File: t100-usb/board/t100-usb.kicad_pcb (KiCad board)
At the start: 2 copper layers, 34.5 x 99.5 mm, 36 parts, among them J1 Conn_01x02_Female, J2 USB_B_Micro, J3 T100-OUT, U1 FR8205, U2 FR8205, U3 ATSAMD11C14A-SS, X1 SWD

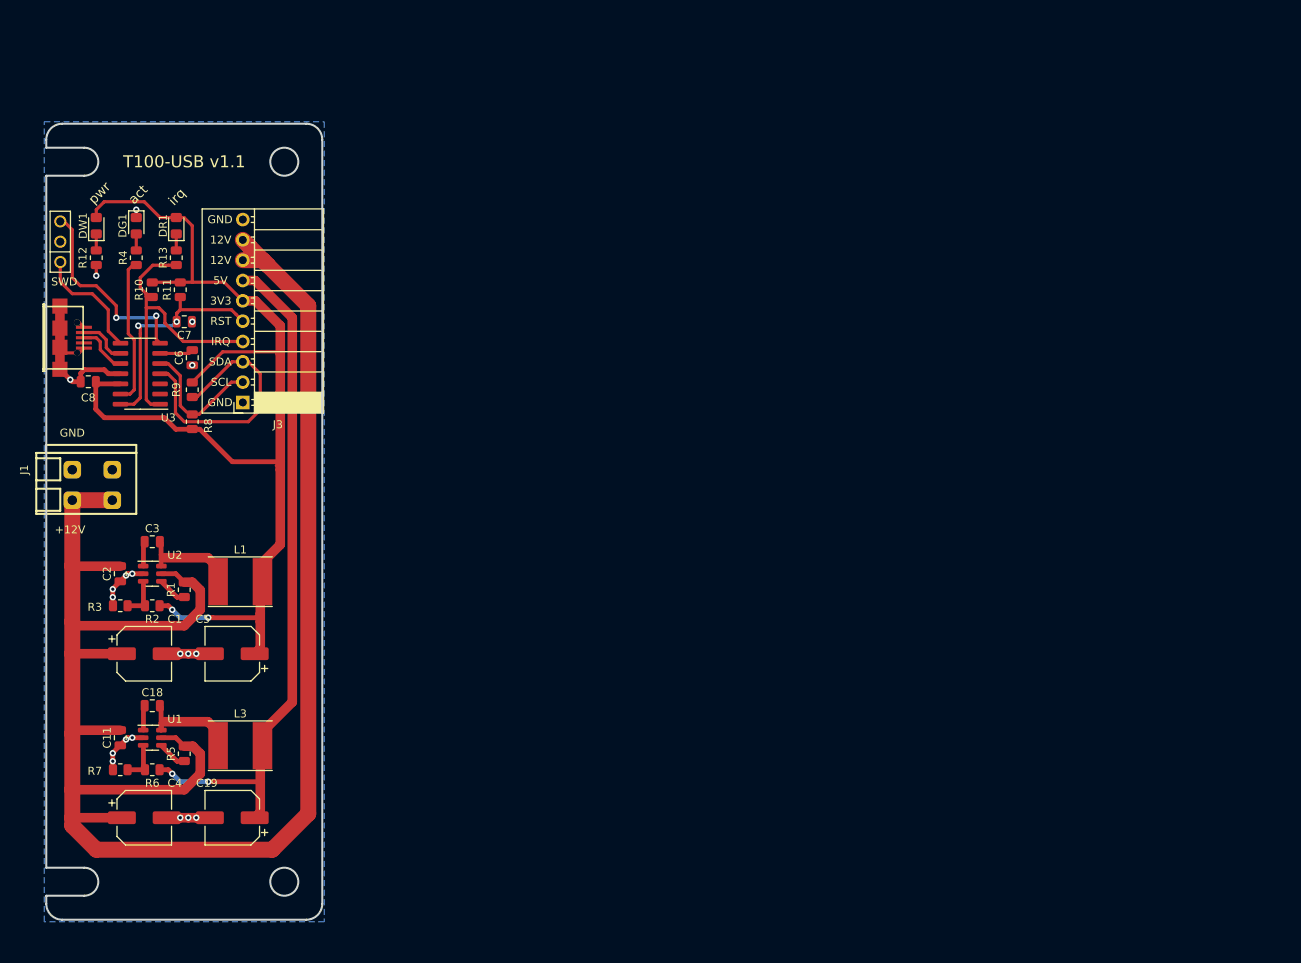
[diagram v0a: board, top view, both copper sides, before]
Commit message: WIP
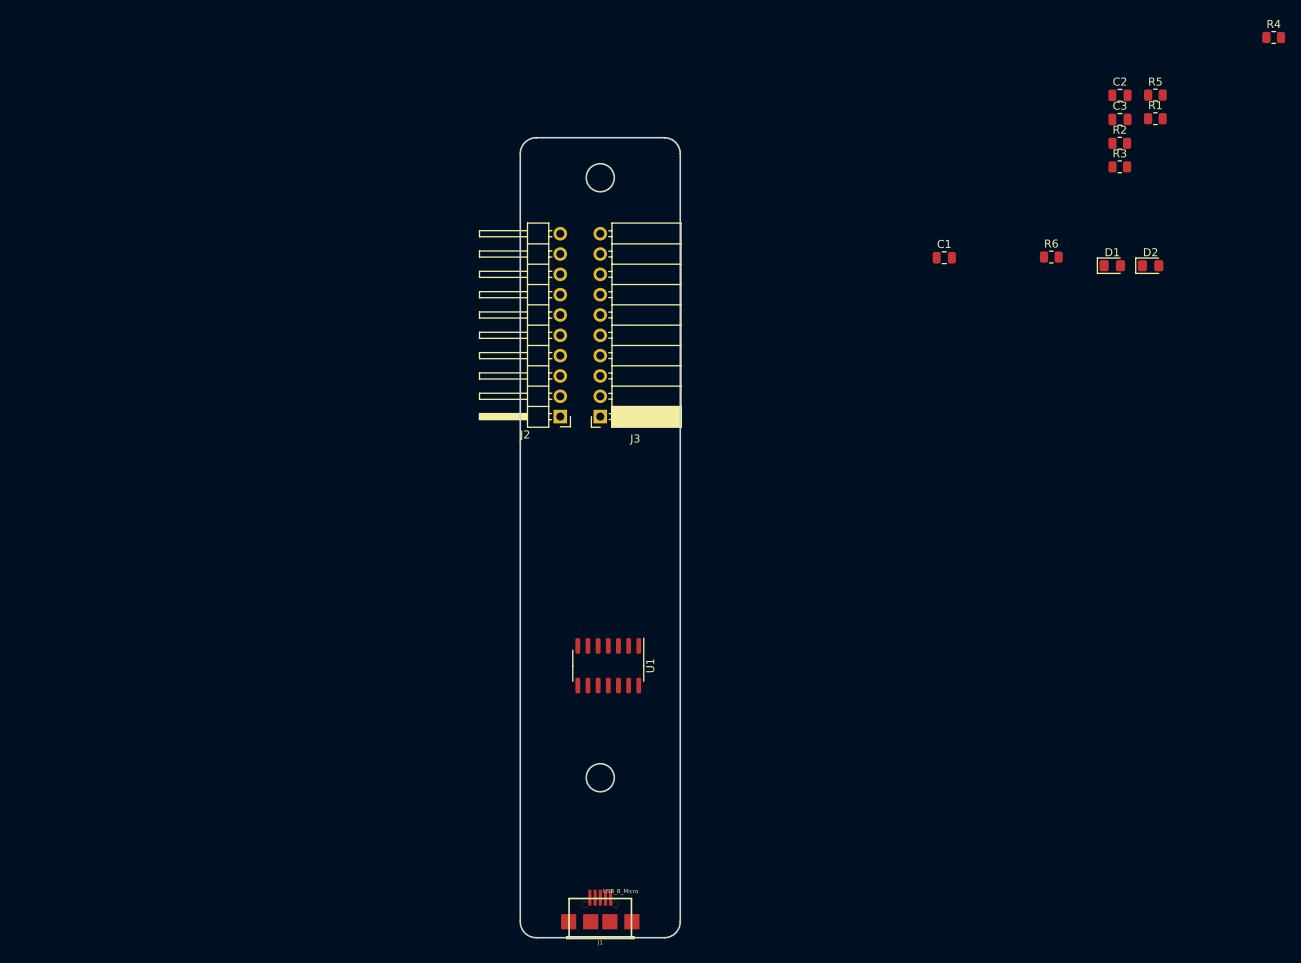
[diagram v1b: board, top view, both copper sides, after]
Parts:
- removed C11, C18, C6, C7, C8: 100n, Capacitor_SMD:C_0805_2012Metric
- removed C19, C4, C5: 100u/12V, Capacitor_SMD:CP_Elec_6.3x5.4
- removed DG1: GREEN, LED_SMD:LED_0805_2012Metric_Pad1.15x1.40mm_HandSolder
- removed DR1: RED, LED_SMD:LED_0805_2012Metric_Pad1.15x1.40mm_HandSolder
- removed DW1: WHITE, LED_SMD:LED_0805_2012Metric_Pad1.15x1.40mm_HandSolder
- removed L1, L3: 6.8uH, Drake:CKCS6028
- removed R10, R11, R8, R9: 1K5, Resistor_SMD:R_0805_2012Metric
- removed R12: 1k5, Resistor_SMD:R_0805_2012Metric
- removed R13: 270R, Resistor_SMD:R_0805_2012Metric
- removed R7: 4.22k 1%, Resistor_SMD:R_0805_2012Metric
- removed U2: FR8205, Package_TO_SOT_SMD:SOT-23-6
- removed U3: ATSAMD11C14A-SS, Package_SO:SOIC-14_3.9x8.7mm_P1.27mm
- removed X1: SWD, Drake:SWD
- added D1: GREEN, LED_SMD:LED_0805_2012Metric_Pad1.15x1.40mm_HandSolder, F.Cu at (216.0, 68.0)
- added D2: RED, LED_SMD:LED_0805_2012Metric_Pad1.15x1.40mm_HandSolder, F.Cu at (220.8, 68.0)
- C1: value 100u/12V -> 100n; footprint Capacitor_SMD:CP_Elec_6.3x5.4 -> Capacitor_SMD:C_0805_2012Metric
- J1: value Conn_01x02_Female -> USB_B_Micro; footprint Drake:DG235-3.81-02P -> Drake:conn_usb_B_micro_smd-2
- J2: value USB_B_Micro -> T100-IN; footprint Drake:conn_usb_B_micro_smd-2 -> Connector_PinHeader_2.54mm:PinHeader_1x10_P2.54mm_Horizontal
- R1: value 100k -> 1K5
- R2: value 30k 1% -> 1K5
- R3: value 6.65k 1% -> 1K5
- R4: value 270R -> 1K5
- R5: value 100k -> 270R
- R6: value 30.9k 1% -> 270R
- U1: value FR8205 -> ATSAMD11C14A-SS; footprint Package_TO_SOT_SMD:SOT-23-6 -> Package_SO:SOIC-14_3.9x8.7mm_P1.27mm
- moved R5 146.7 mm to (221.4, 46.7), turned to 0 degrees
- moved R4 144.8 mm to (236.2, 39.5), turned to 0 degrees
- moved C2 138.5 mm to (217.0, 46.7), turned to 0 degrees
- moved R3 136.5 mm to (216.9, 55.6)
- moved R1 134.9 mm to (221.4, 49.6), turned to 0 degrees
- moved R2 134.0 mm to (216.9, 52.7)
- moved C3 132.0 mm to (217.0, 49.7)
- moved R6 129.4 mm to (208.4, 66.9)
- moved C1 111.6 mm to (195.0, 67.0)
- moved J1 83.1 mm to (152.0, 150.0), turned to 0 degrees
- moved J2 63.3 mm to (147.0, 86.9), turned to 180 degrees
- moved U1 57.7 mm to (153.0, 118.0), turned to -90 degrees
- moved J3 44.7 mm to (152.0, 86.9)
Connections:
- C1 pad 1: +12V -> GND
- C1 pad 2: GND -> +3V3
- C2 pad 2: +12V -> Net-(C2-Pad2)
- C3 pad 1: Net-(C3-Pad1) -> GND
- C3 pad 2: Net-(C3-Pad2) -> /RST
- J1 pad 1: GND -> unconnected-(J1-Pad1)
- J1 pad 2: +12V -> /USB_DM
- J2 pad 1: unconnected-(J2-Pad1) -> GND
- J2 pad 2: /USB_DM -> /SCL
- J2 pad 3: /USB_DP -> /SDA
- J2 pad 4: unconnected-(J2-Pad4) -> /IRQ
- J2 pad 5: GND -> /RST
- J2 pad 6: GND -> +3V3
- R1 pad 1: Net-(R1-Pad1) -> /SCL
- R1 pad 2: +12V -> +3V3
- R2 pad 1: Net-(R2-Pad1) -> /SDA
- R3 pad 1: GND -> /IRQ
- R3 pad 2: Net-(R2-Pad1) -> +3V3
- R4 pad 1: /I2C_ACT -> /RST
- R4 pad 2: Net-(DG1-Pad2) -> +3V3
- R5 pad 1: Net-(R5-Pad1) -> /I2C_ACT
- R5 pad 2: +12V -> Net-(D1-Pad2)
- R6 pad 1: Net-(R6-Pad1) -> /IRQ
- R6 pad 2: +5V -> Net-(D2-Pad1)
- U1 pad 1: Net-(C18-Pad1) -> /IRQ
- U1 pad 2: GND -> unconnected-(U1-Pad2)
- U1 pad 3: Net-(R6-Pad1) -> unconnected-(U1-Pad3)
- U1 pad 4: Net-(R5-Pad1) -> /SDA
- U1 pad 5: +12V -> /SCL
- U1 pad 6: Net-(C18-Pad2) -> Net-(C2-Pad2)
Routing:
- net +12V: track 231.8 -> 0.00 mm
- net +3V3: track 141.5 -> 0.00 mm, vias 2 -> 0
- net +5V: track 85.7 -> 0.00 mm, vias 2 -> 0
- net GND: track 47.7 -> 0.00 mm, vias 19 -> 0
- net /IRQ: track 38.3 -> 0.00 mm
- net /SDA: track 33.4 -> 0.00 mm
- net /RST: track 28.6 -> 0.00 mm, vias 2 -> 0
- net /SWCLK: track 25.1 -> 0.00 mm, vias 2 -> 0
- net /I2C_ACT: track 18.5 -> 0.00 mm
- net /SCL: track 16.0 -> 0.00 mm
- net /SWDIO: track 14.7 -> 0.00 mm
- net Net-(C18-Pad2): track 13.5 -> 0.00 mm
- net Net-(C3-Pad2): track 12.1 -> 0.00 mm
- net /USB_DP: track 6.49 -> 0.00 mm
- net /USB_DM: track 6.24 -> 0.00 mm
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- removed copper zone on B.Cu, net GND
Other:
- board size 34.5 x 99.5 mm -> 20 x 100 mm
- rule pad_to_mask_clearance: 0.051 -> 0
- board text removed: "+12V"
- board text removed: "12V"
- board text removed: "3V3"
- board text removed: "5V"
- board text removed: "GND"
- board text removed: "IRQ"
- board text removed: "RST"
- board text removed: "SCL"
- board text removed: "SDA"
- board text removed: "SWD"
- board text removed: "T100-USB v1.1"
- board text removed: "act"
- board text removed: "irq"
- board text removed: "pwr"
